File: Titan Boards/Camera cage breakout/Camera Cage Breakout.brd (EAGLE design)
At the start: 57.1 x 63.5 mm, 5 parts

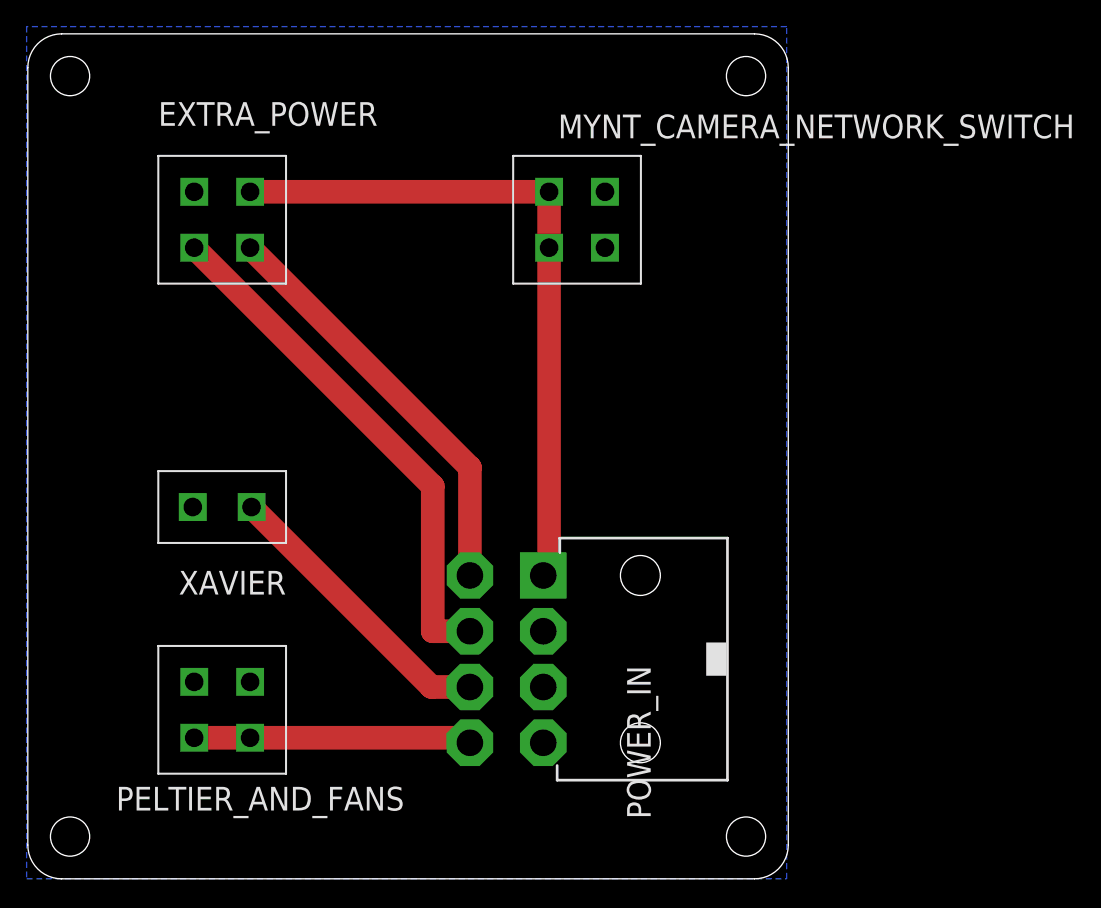
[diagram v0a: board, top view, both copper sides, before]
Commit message: final camera cage breakout with gerbers
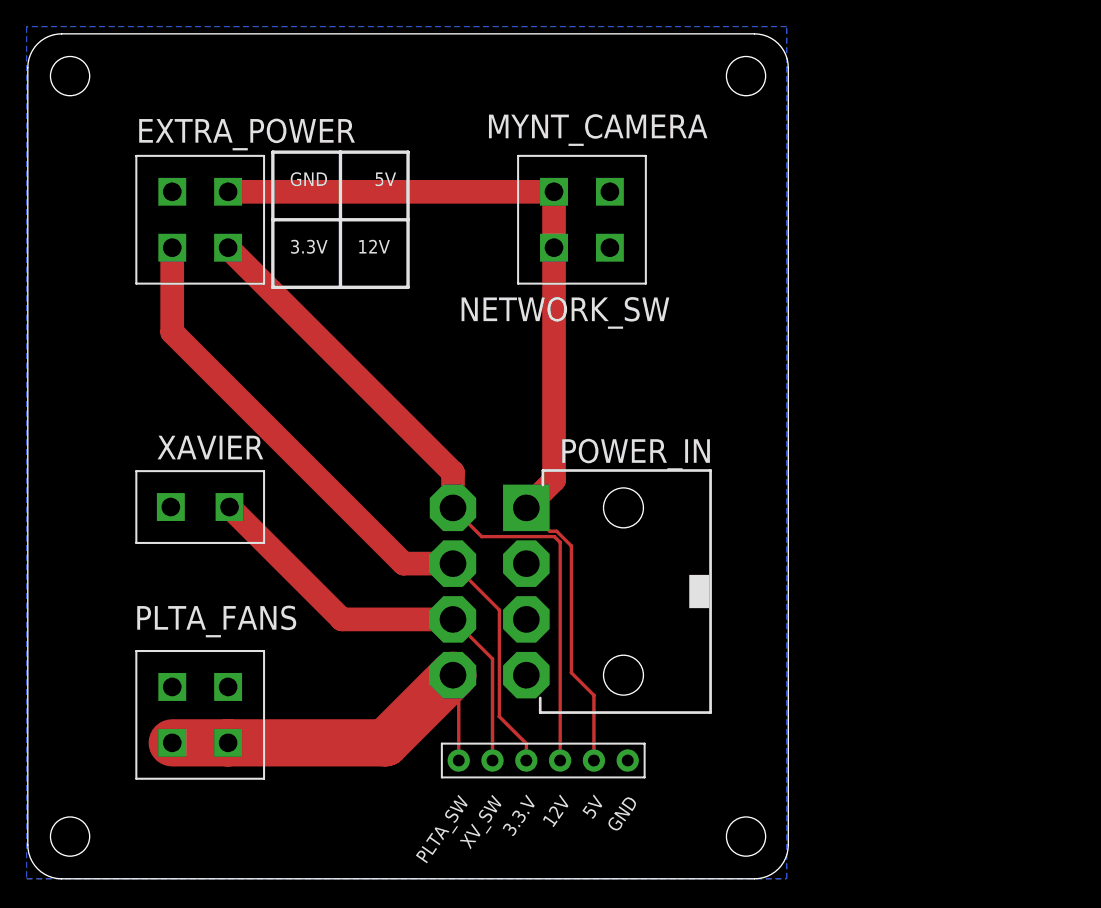
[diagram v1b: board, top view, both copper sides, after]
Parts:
- removed MYNT_CAMERA_NETWORK_SWITCH, PELTIER_AND_FANS: 4PIN-VERT, Vertical_Connectors:4PIN-VERT
- added MYNT_CAMERA, PLTA_FANS: 4PIN-VERT, Vertical_Connectors:4PIN-VERT
- added U$1: CAMERA_CAGE_TEST, 3M_929852_Connector:6-PIN
- moved POWER_IN 5.24 mm to (48.3, 36.8)
- moved EXTRA_POWER 1.65 mm to (23.7, 64.8)
- moved XAVIER 1.65 mm to (23.7, 43.2)
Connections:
- net 12V: now also U$1.P$3
- net 3.3V: now also U$1.P$4
- net 5V: now also MYNT_CAMERA.P$1, MYNT_CAMERA.P$2, U$1.P$2; no longer MYNT_CAMERA_NETWORK_SWITCH.P$1, MYNT_CAMERA_NETWORK_SWITCH.P$2
- net GND: now also MYNT_CAMERA.P$3, MYNT_CAMERA.P$4, PLTA_FANS.P$3, PLTA_FANS.P$4, U$1.P$1; no longer MYNT_CAMERA_NETWORK_SWITCH.P$3, MYNT_CAMERA_NETWORK_SWITCH.P$4, PELTIER_AND_FANS.P$3, PELTIER_AND_FANS.P$4
- net PELTIER_SWITCHED: now also PLTA_FANS.P$1, PLTA_FANS.P$2, U$1.P$6; no longer PELTIER_AND_FANS.P$1, PELTIER_AND_FANS.P$2
- net XAVIER_SWITCHED: now also U$1.P$5
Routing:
- net 12V: track 31.5 -> 52.1 mm
- net 5V: track 51.5 -> 70.5 mm
- net 3.3V: track 39.0 -> 51.7 mm
- net XAVIER_SWITCHED: track 22.0 -> 32.1 mm
- net PELTIER_SWITCHED: track 20.9 -> 29.8 mm
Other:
- board text added: "12V"
- board text added: "3.3.V"
- board text added: "3.3V"
- board text added: "5V"
- board text added: "GND"
- board text added: "NETWORK_SW"
- board text added: "PLTA_SW"
- board text added: "XV_SW"
